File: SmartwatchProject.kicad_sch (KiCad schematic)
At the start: 30 parts, among them J1 USB_B_Micro, J2 SM13B-GHS-TB_LF__SN_, SW1 SW_Push, SW2 SW_Push, U1 ESP32-S3-WROOM-1, U2 DS3231M, U3 ADXL345BCCZ, U4 DRV2605LDGSR, U6 MAX98357A, U8 AMS1117-3.3, U9 MCP73831-2-MC

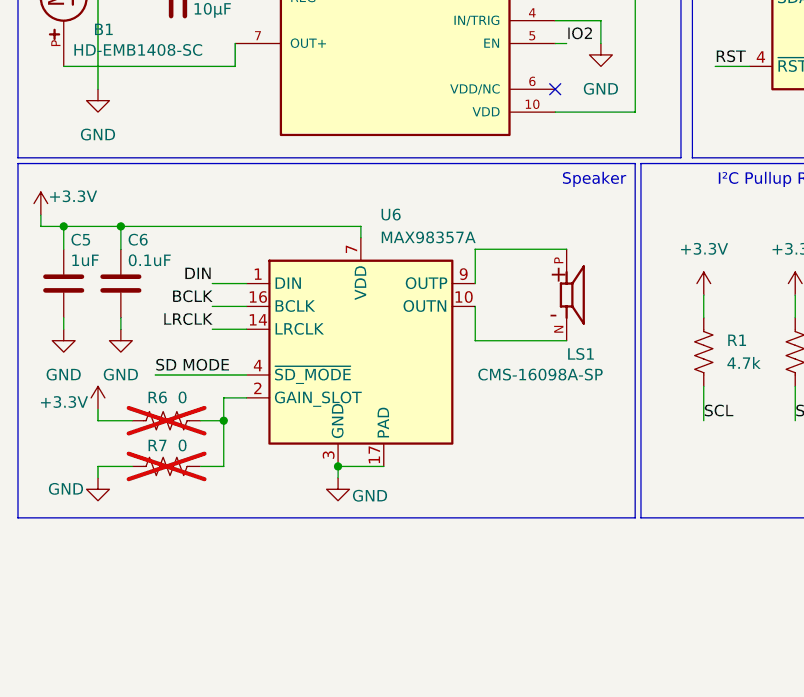
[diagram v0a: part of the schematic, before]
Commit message: SixthCommit
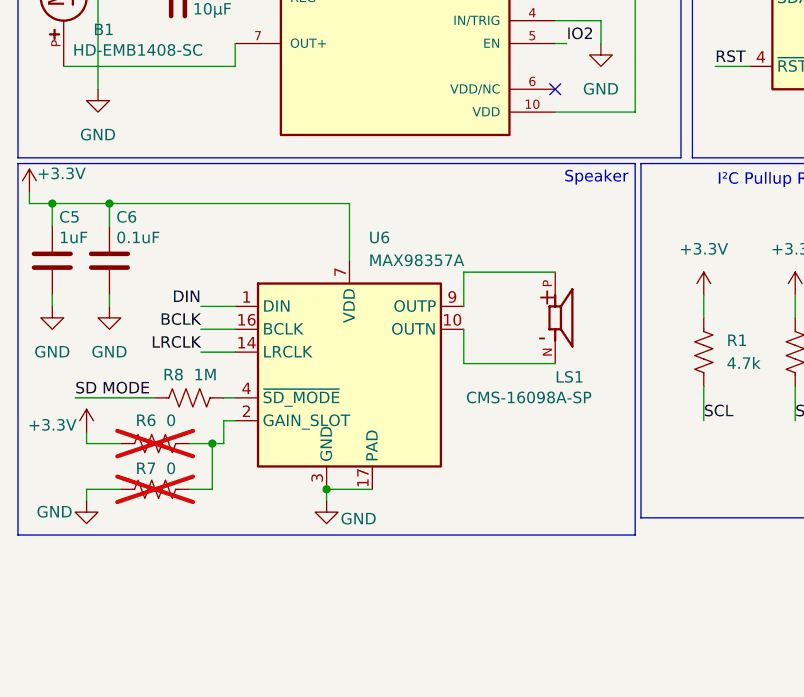
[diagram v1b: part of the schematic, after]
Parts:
- added R8: 1M, symbol Device:R_US
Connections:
- net SD MODE: now also R8.1; no longer U6.4 (~{SD_MODE})
- new net: R8.2, U6.4 (~{SD_MODE})
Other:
- moved on the sheet: C5, C6, LS1, R6, R7, U6
